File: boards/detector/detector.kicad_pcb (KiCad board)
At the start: 2 copper layers, 130 x 130 mm, 15 parts, among them Q1 MMBT3906, Q2 MMBT3904, SW1 Button, U1 ESP32

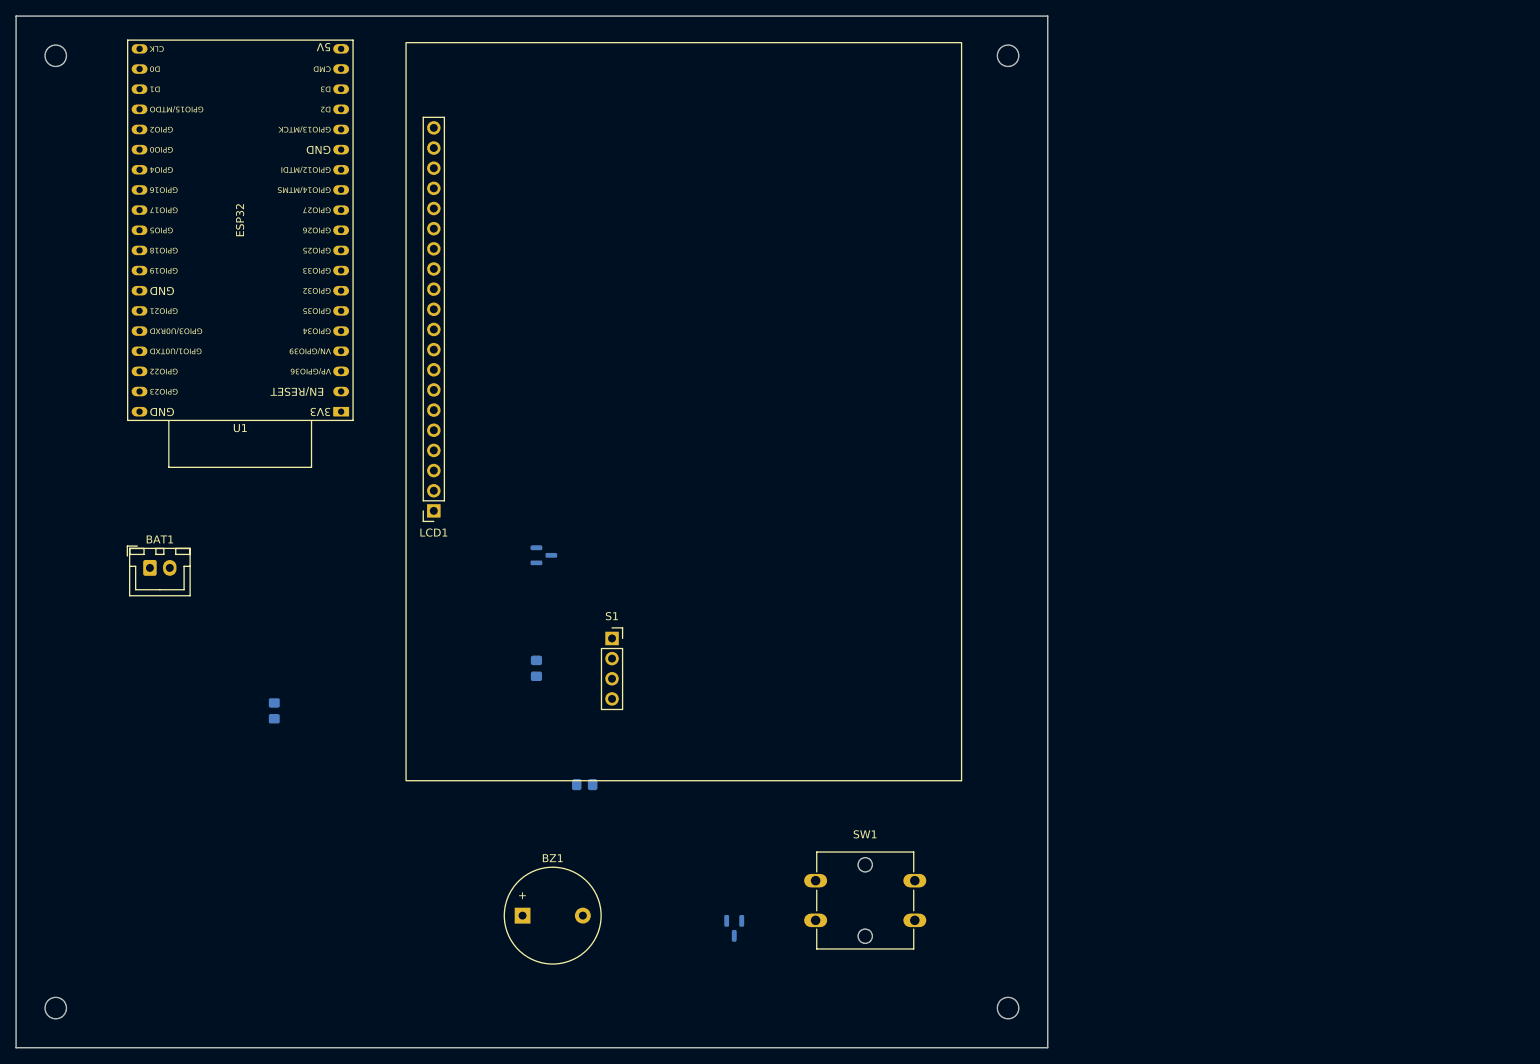
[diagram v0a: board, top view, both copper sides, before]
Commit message: more work done on the detector board
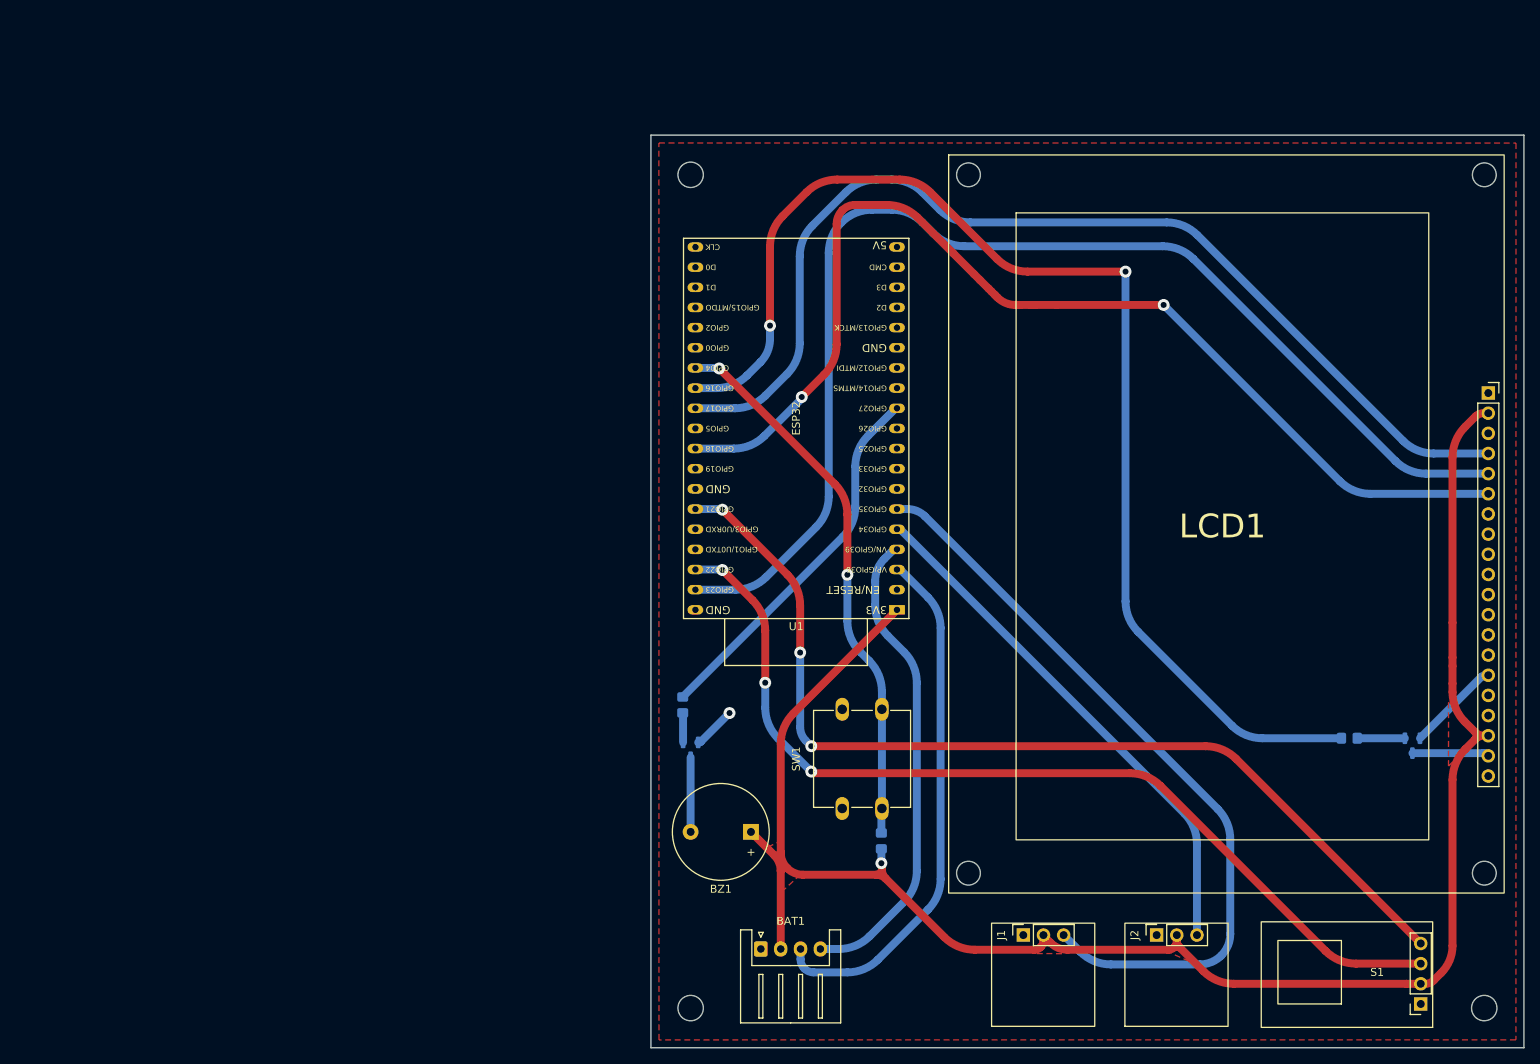
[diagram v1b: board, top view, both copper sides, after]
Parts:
- removed the REF** at (145.0, 145.0)
- removed the REF** at (145.0, 25.0)
- removed the REF** at (25.0, 145.0)
- removed the REF** at (25.0, 25.0)
- added HOLE1: MountingHole_3.2mm_M3, MountingHole:MountingHole_3.2mm_M3, F.Cu at (105.0, 40.0)
- added HOLE3: MountingHole_3.2mm_M3, MountingHole:MountingHole_3.2mm_M3, F.Cu at (105.0, 145.0)
- added HOLE4: MountingHole_3.2mm_M3, MountingHole:MountingHole_3.2mm_M3, F.Cu at (205.0, 145.0)
- added J1: CO, Library:DFRobot Sensor, F.Cu at (146.9, 135.8)
- added J2: Smoke, Library:DFRobot Sensor, F.Cu at (163.7, 135.8)
- added REF**: KiCad-Logo2_12mm_SilkScreen, Symbol:KiCad-Logo2_12mm_SilkScreen, B.Cu at (154.9, 114.3)
- added REF**: OSHW-Logo_19x20mm_SilkScreen, Symbol:OSHW-Logo_19x20mm_SilkScreen, B.Cu at (154.9, 78.7)
- BAT1: footprint Connector_JST:JST_XH_B2B-XH-A_1x02_P2.50mm_Vertical -> Connector_JST:JST_XH_S4B-XH-A_1x04_P2.50mm_Horizontal
- Q1: value MMBT3906 -> MMBT2222A
- Q2: value MMBT3904 -> MMBT2222A
- R1, R2, R3: value 1K -> 10KΩ
- S1: footprint Connector_PinSocket_2.54mm:PinSocket_1x04_P2.54mm_Vertical -> Library:SCD41
- SW1: footprint Button_Switch_THT:SW_SPST_Omron_B3F-40xx -> Library:Button
- moved LCD1 133.7 mm to (205.5, 67.5), turned to 0 degrees
- moved Q1 112.0 mm to (195.9, 111.9), turned to -90 degrees
- moved S1 111.8 mm to (197.0, 144.5), turned to 180 degrees
- moved R1 102.8 mm to (188.0, 111.0), turned to 180 degrees
- moved BAT1 90.7 mm to (113.8, 137.6)
- moved U1 74.4 mm to (131.0, 94.8)
- moved R3 51.5 mm to (104.0, 106.8)
- moved R2 38.0 mm to (129.0, 123.9), turned to -90 degrees
- moved BZ1 30.7 mm to (112.6, 122.8), turned to 180 degrees
- moved Q2 23.2 mm to (105.0, 112.5)
- moved SW1 9.69 mm to (124.1, 119.8), turned to 90 degrees
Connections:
- BAT1 pad 1: VCC -> GND
- BAT1 pad 2: GND -> VCC
- LCD1 pad 18: unconnected-(LCD1-VOUT-Pad18) -> VCC
- LCD1 pad 20: GND -> unconnected-(LCD1-BLK-Pad20)
- Q1 pad 2: VCC -> GND
- R1 pad 1: /BACKLIGHT -> Net-(Q1-B)
- R1 pad 2: Net-(Q1-B) -> /BACKLIGHT
- S1 pad 1: /I2C SDA -> GND
- S1 pad 2: /I2C SCL -> VCC
- S1 pad 3: VCC -> /I2C SCL
- S1 pad 4: GND -> /I2C SDA
- U1 pad 3: unconnected-(U1-SENSOR_VP/GPIO36/ADC1_CH0-Pad3) -> /REF ON
- U1 pad 4: unconnected-(U1-SENSOR_VN/GPIO39/ADC1_CH3-Pad4) -> /REF BAT
- U1 pad 5: unconnected-(U1-VDET_1/GPIO34/ADC1_CH6-Pad5) -> /SMOKE
- U1 pad 6: unconnected-(U1-VDET_2/GPIO35/ADC1_CH7-Pad6) -> /CO
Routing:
- net VCC: track 0.00 -> 232.6 mm, vias 0 -> 1
- net /BACKLIGHT: track 0.00 -> 154.2 mm, vias 0 -> 2
- net /R/W: track 0.00 -> 152.0 mm
- net /E: track 0.00 -> 137.2 mm, vias 0 -> 2
- net /RS: track 0.00 -> 133.1 mm
- net /I2C SDA: track 0.00 -> 124.3 mm, vias 0 -> 3
- net /I2C SCL: track 0.00 -> 119.2 mm, vias 0 -> 3
- net /CO: track 0.00 -> 96.5 mm
- net /BUTTON: track 0.00 -> 69.3 mm, vias 0 -> 2
- net /REF ON: track 0.00 -> 66.8 mm
- net /SMOKE: track 0.00 -> 66.7 mm
- net /REF BAT: track 0.00 -> 60.4 mm
- net /BUZZER: track 0.00 -> 47.1 mm
- net GND: track 0.00 -> 17.3 mm, vias 0 -> 1
- net Net-(LCD1-BLA): track 0.00 -> 9.67 mm
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- added copper zone on F.Cu, net GND
- added copper zone on F.Cu, net VCC
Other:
- board size 130 x 130 mm -> 110 x 115 mm
